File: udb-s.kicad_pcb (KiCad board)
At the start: 4 copper layers, 40 x 9 mm, 11 parts, among them J1 TYPE-C-31-M-12, J2 78171-0004, U1 TPD4E05U06DQAR

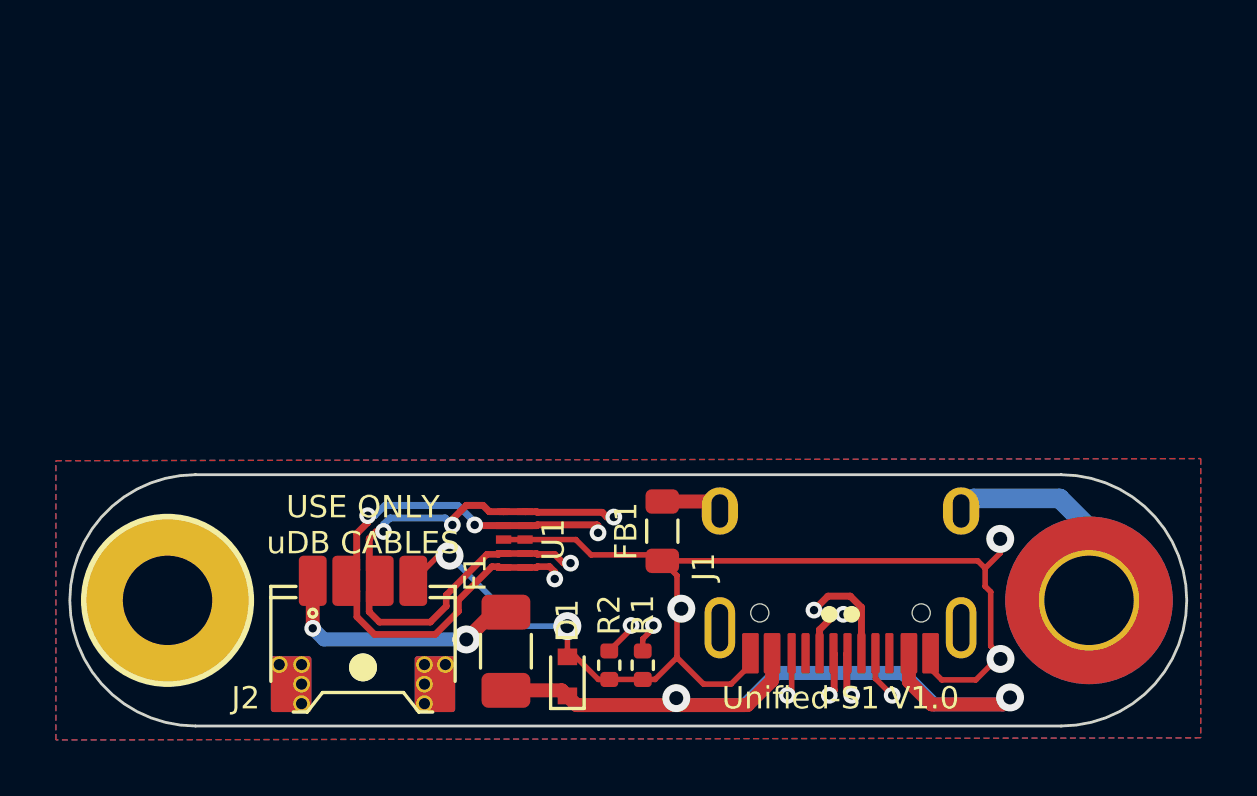
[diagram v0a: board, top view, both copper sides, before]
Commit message: Lil-CC init upload
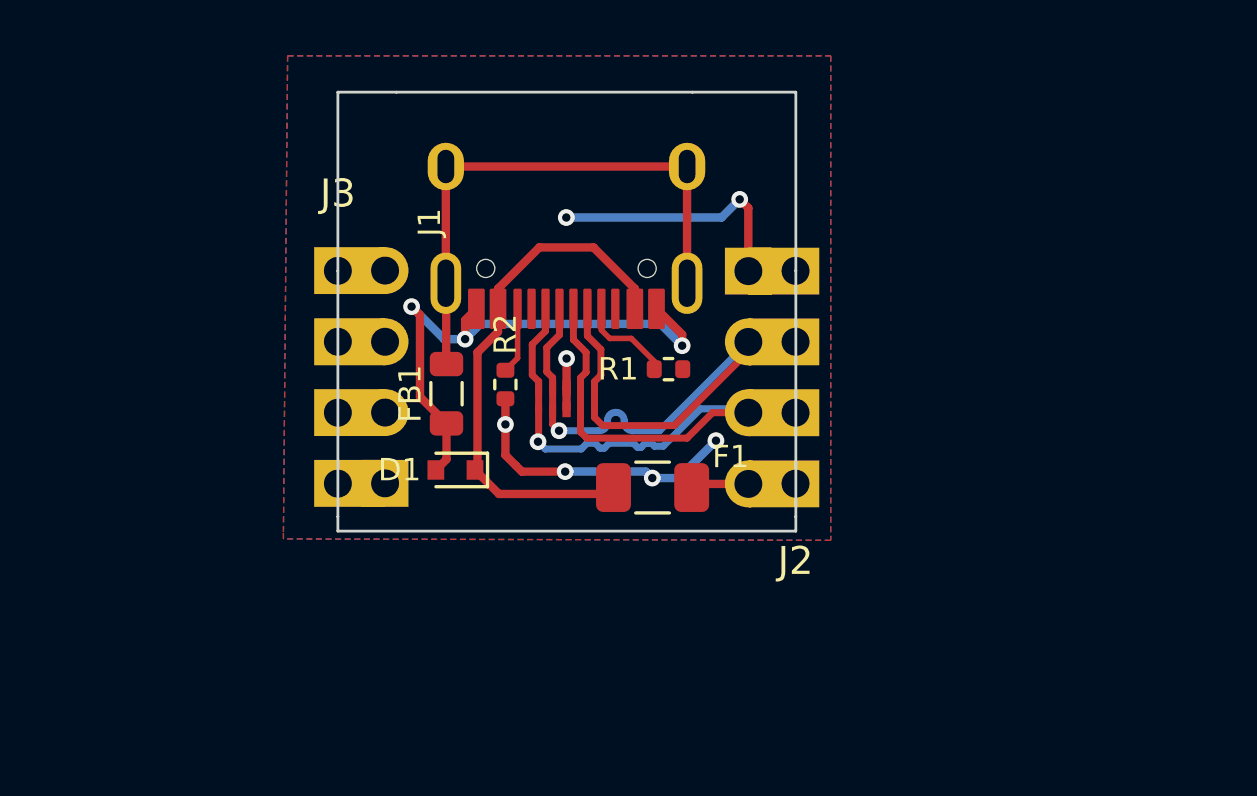
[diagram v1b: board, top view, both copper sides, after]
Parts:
- removed G***: LOGO, locallib:UnifiedLogo
- removed H1: MountingHole, MountingHole:MountingHole_3.2mm_M3_DIN965_Pad_TopBottom
- removed H2: MountingHole, MountingHole:MountingHole_3.2mm_M3_DIN965_Pad_TopOnly
- added J3: Conn_01x04, acheron_Connectors:Castellated2.54-01x04, F.Cu at (121.1, 83.2)
- J2: value 78171-0004 -> Conn_01x04; footprint locallib:PicoEZMate-Reinforced-Lite -> acheron_Connectors:Castellated2.54-01x04
- moved J2 16.5 mm to (137.5, 90.8), turned to 180 degrees
- moved J1 15.8 mm to (129.3, 76.9)
- moved R2 10.7 mm to (127.1, 87.3)
- moved R1 10.6 mm to (132.9, 86.7), turned to 180 degrees
- moved FB1 9.16 mm to (125.0, 87.6)
- moved D1 8.41 mm to (125.3, 90.3), turned to 180 degrees
- moved F1 7.87 mm to (132.4, 91.0), turned to 0 degrees
- moved U1 5.38 mm to (129.3, 87.8), turned to 90 degrees
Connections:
- J2 pad 2: D- -> D+
- J2 pad 3: D+ -> D-
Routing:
- net D-: track 49.1 -> 24.8 mm, vias 6 -> 1
- net D+: track 47.9 -> 24.9 mm, vias 6 -> 1
- net VBUS: track 30.0 -> 19.2 mm, vias 2 -> 0
- net GND: track 51.4 -> 41.7 mm, vias 6 -> 10
- net Net-(J1-PadA5): track 12.4 -> 3.40 mm, vias 2 -> 0
- net GNDPWR: track 10.9 -> 19.9 mm
- net 5V: track 9.19 -> 1.95 mm, vias 2 -> 0
- net Net-(J1-PadB5): track 9.50 -> 2.38 mm, vias 2 -> 0
- removed copper zone on In1.Cu, net GND
- removed copper zone on In2.Cu, net GND
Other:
- board size 40 x 9 mm -> 16.4 x 15.7 mm
- copper layers 4 -> 2
- board text removed: "USE ONLY uDB CABLES"
- board text removed: "Unified-S1 V1.0"
- board text removed: "Unified-S1 V1.0 www.unified- daughterboard.github.io"
